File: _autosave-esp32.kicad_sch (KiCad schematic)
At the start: 47 parts, among them J2 Conn_01x05, SW1 Reset, SW2 BOOT, U6 ESP32-S3R8, U7 W25Q128JVSIQ, Y1 40MHz

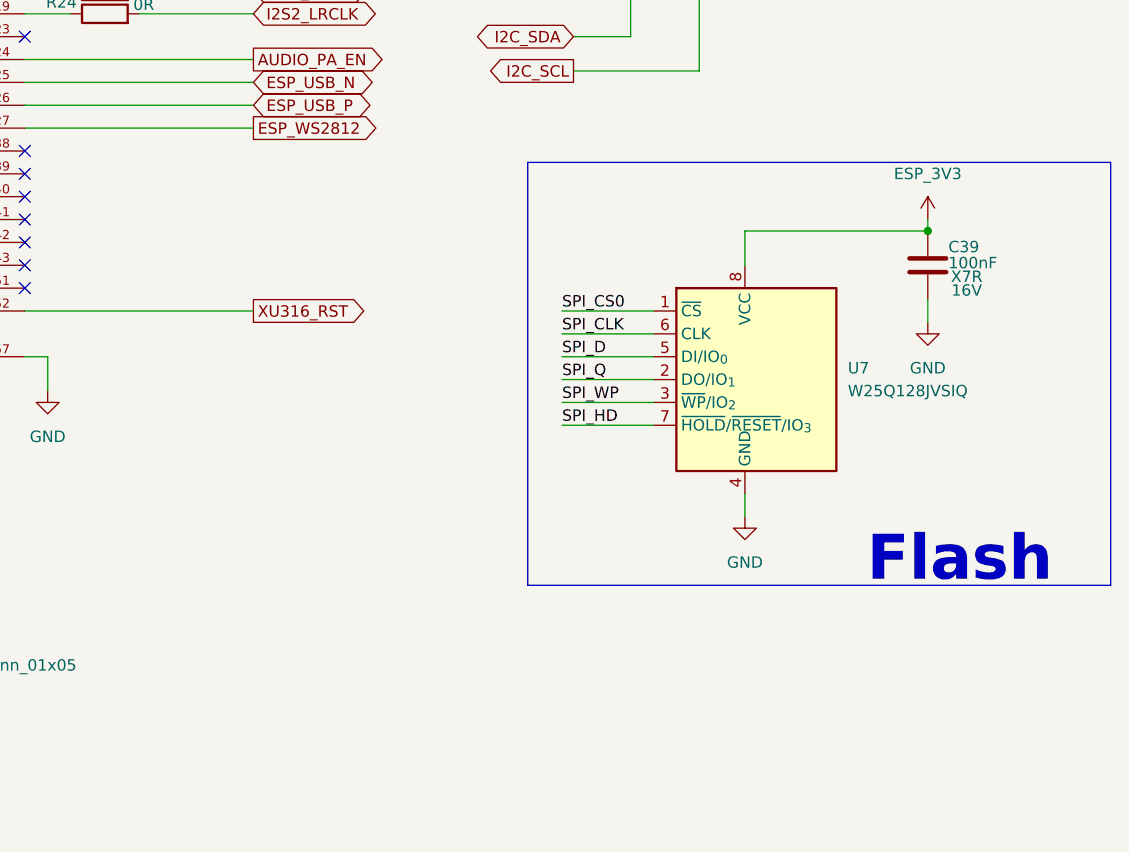
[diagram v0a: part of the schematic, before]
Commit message: complete redesign
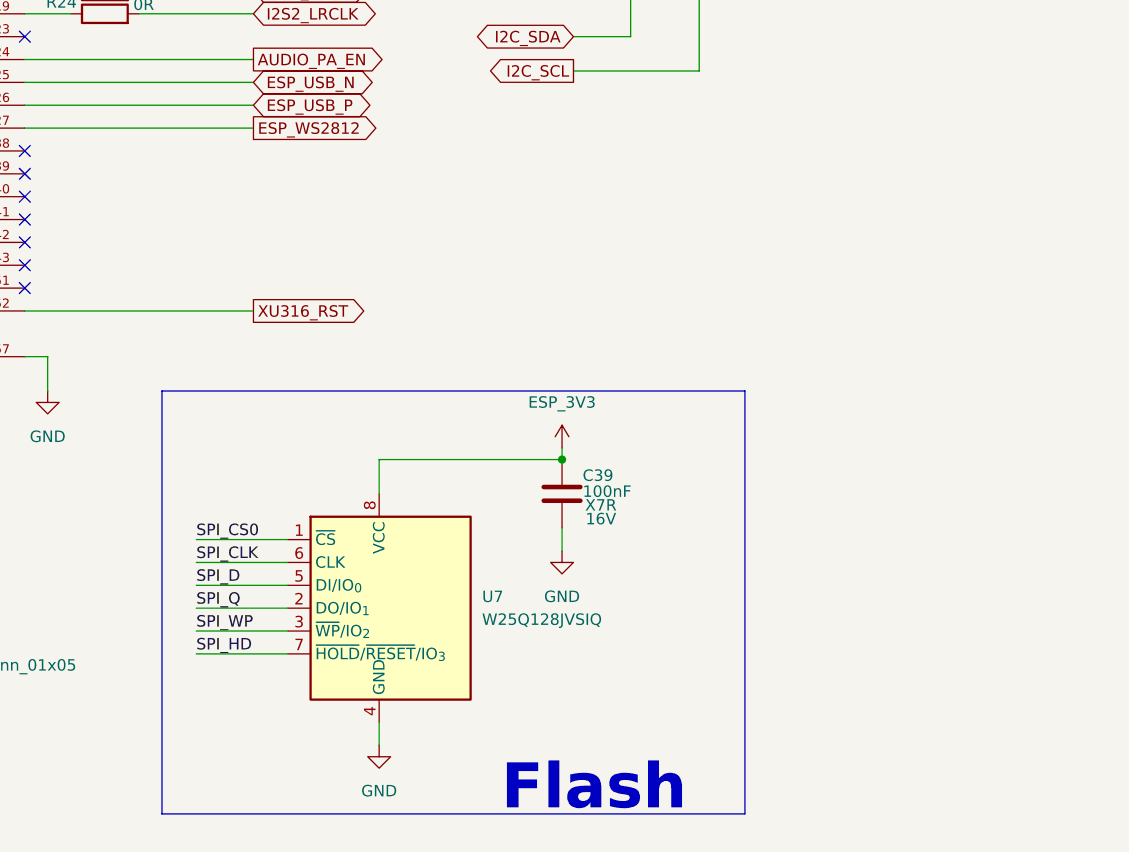
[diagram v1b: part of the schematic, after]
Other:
- moved on the sheet: C39, U7
